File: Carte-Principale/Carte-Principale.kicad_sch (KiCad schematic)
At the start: 1 part, among them U1 NUCLEOH723ZG

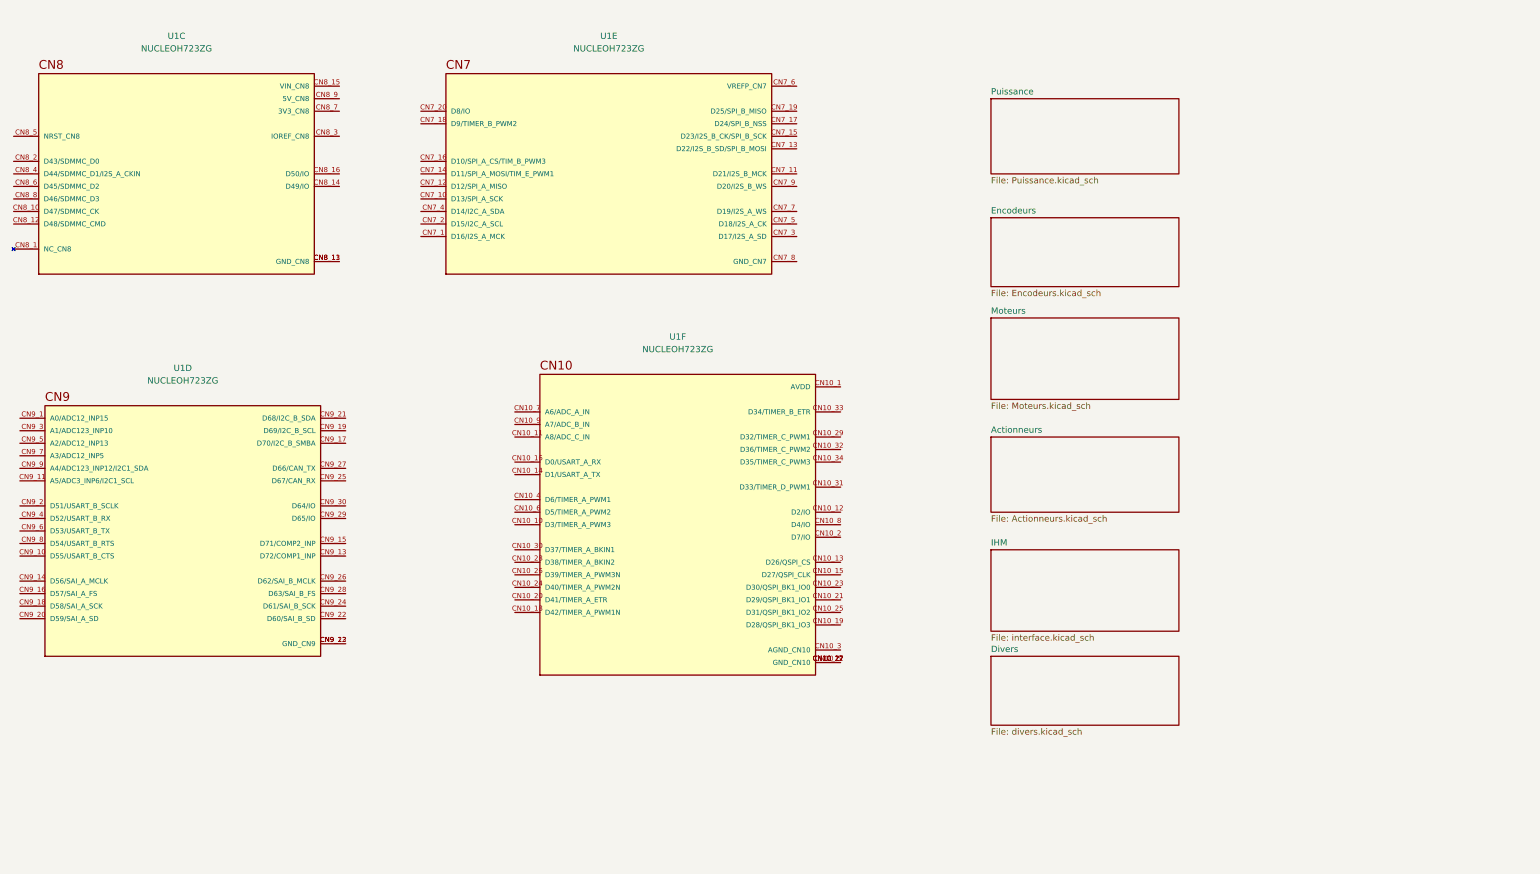
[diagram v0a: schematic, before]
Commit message: Moteurs + Encodeurs
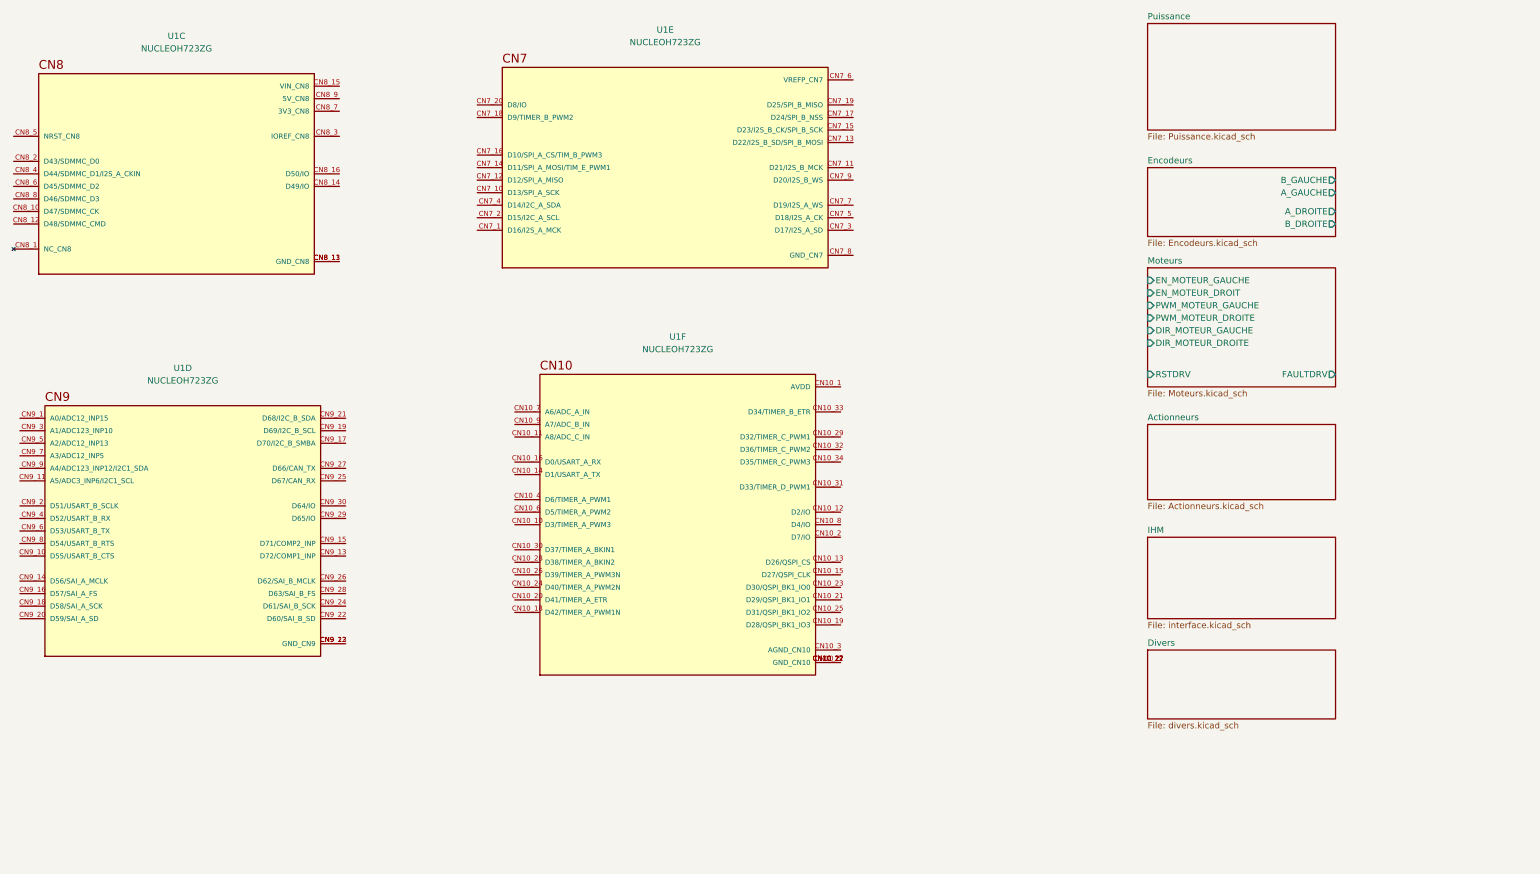
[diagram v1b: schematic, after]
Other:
- sheet Encodeurs ports: added A_DROITE, A_GAUCHE, B_DROITE, B_GAUCHE; removed none
- sheet Moteurs ports: added DIR_MOTEUR_DROITE, DIR_MOTEUR_GAUCHE, EN_MOTEUR_DROIT, EN_MOTEUR_GAUCHE, FAULTDRV, PWM_MOTEUR_DROITE, PWM_MOTEUR_GAUCHE, RSTDRV; removed none
- moved on the sheet: U1E

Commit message: Avancée Actionneur
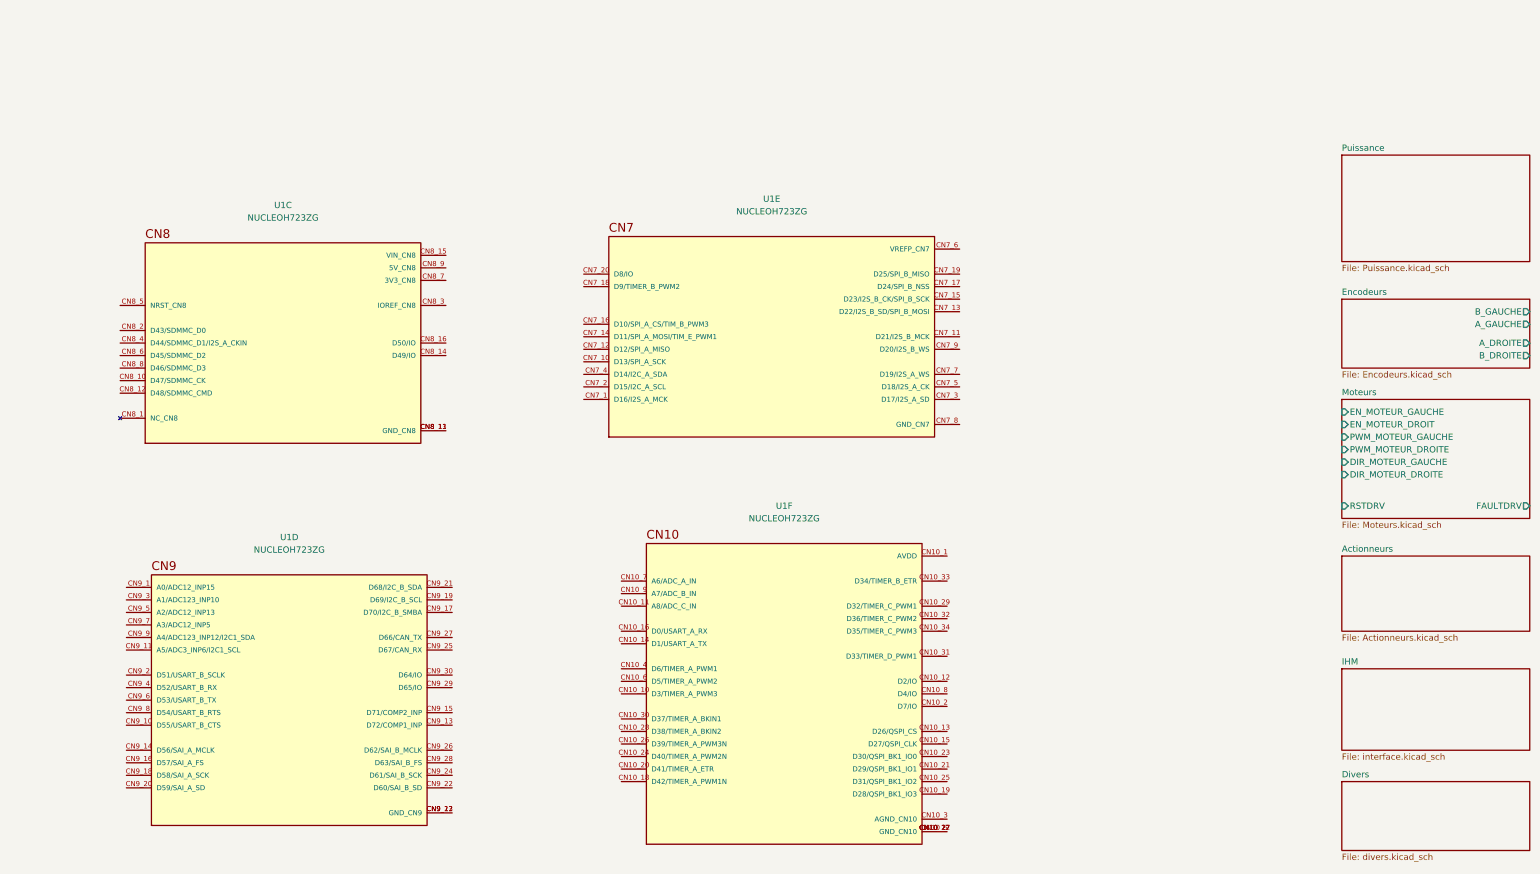
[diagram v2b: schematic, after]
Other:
- moved on the sheet: U1C, U1D, U1E, U1F
